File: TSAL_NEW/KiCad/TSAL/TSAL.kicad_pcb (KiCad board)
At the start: 2 copper layers, 101.6 x 25.4 mm, 0 parts

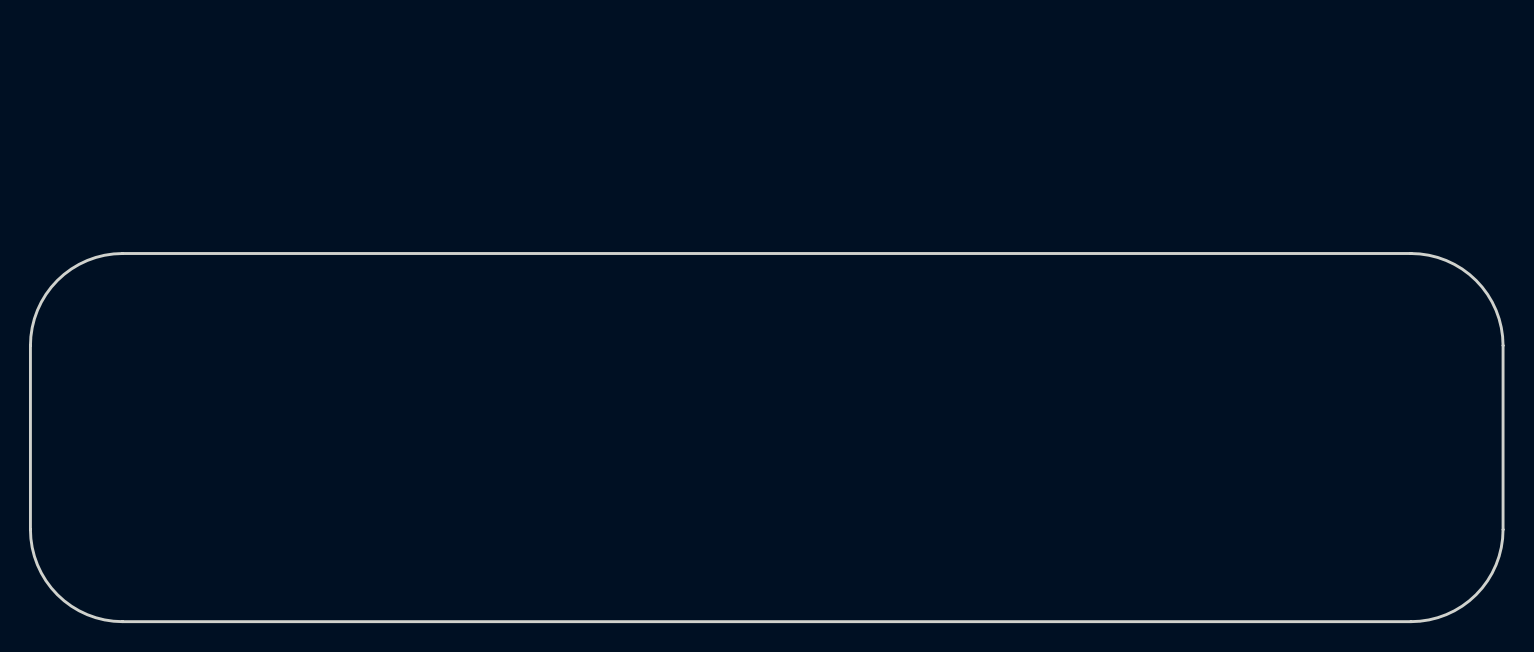
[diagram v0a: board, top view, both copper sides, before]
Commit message: Ready for Review
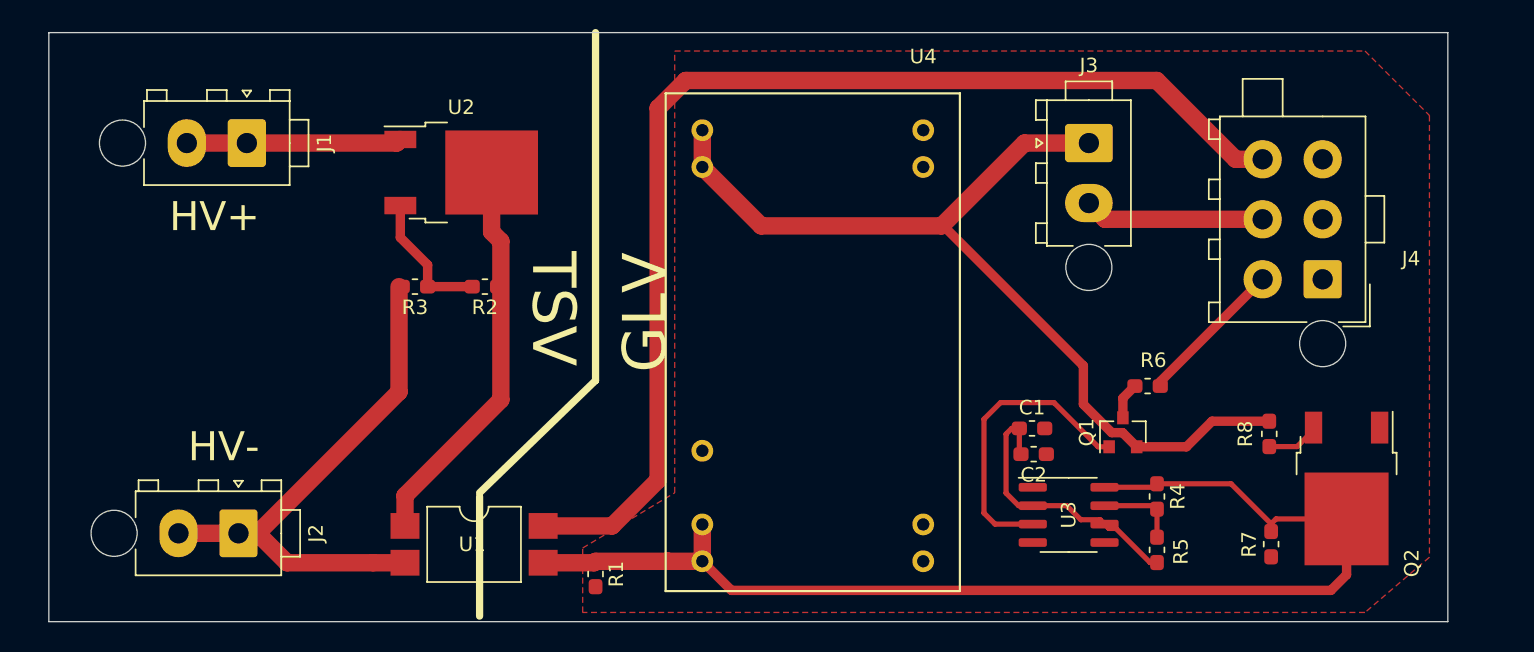
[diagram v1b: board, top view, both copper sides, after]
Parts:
- added C1: 1u, Capacitor_SMD:C_0603_1608Metric_Pad1.05x0.95mm_HandSolder, F.Cu at (174.5, 113.7)
- added C2: 1u, Capacitor_SMD:C_0603_1608Metric_Pad1.05x0.95mm_HandSolder, F.Cu at (174.6, 115.4)
- added J1: HV INPUT, Connector_TE-Connectivity:TE_MATE-N-LOK_1-770866-x_1x02_P4.14mm_Vertical, F.Cu at (120.3, 94.0)
- added J2: HV GND, Connector_TE-Connectivity:TE_MATE-N-LOK_1-770866-x_1x02_P4.14mm_Vertical, F.Cu at (119.8, 120.9)
- added J3: Green_LED_Jp, Connector_TE-Connectivity:TE_MATE-N-LOK_1-770866-x_1x02_P4.14mm_Vertical, F.Cu at (178.4, 94.0)
- added J4: Conn_02x03_Counter_Clockwise, Connector_TE-Connectivity:TE_MATE-N-LOK_1-770875-x_2x03_P4.14mm_Vertical, F.Cu at (194.6, 103.4)
- added Q1: BSS84, Package_TO_SOT_SMD:SOT-23, F.Cu at (180.8, 113.9)
- added Q2: FDD8447L, Package_TO_SOT_SMD:TO-252-2, F.Cu at (196.2, 117.8)
- added R1: 10k, Resistor_SMD:R_0603_1608Metric_Pad1.05x0.95mm_HandSolder, F.Cu at (144.4, 123.7)
- added R2: 180k, Resistor_SMD:R_0603_1608Metric_Pad1.05x0.95mm_HandSolder, F.Cu at (136.8, 103.9)
- added R3: 20k, Resistor_SMD:R_0603_1608Metric_Pad1.05x0.95mm_HandSolder, F.Cu at (131.9, 103.9)
- added R4: 100k, Resistor_SMD:R_0603_1608Metric_Pad1.05x0.95mm_HandSolder, F.Cu at (183.1, 118.4)
- added R5: 235k, Resistor_SMD:R_0603_1608Metric_Pad1.05x0.95mm_HandSolder, F.Cu at (183.1, 122.0)
- added R6: R, Resistor_SMD:R_0603_1608Metric_Pad1.05x0.95mm_HandSolder, F.Cu at (182.5, 110.7)
- added R7: 10k, Resistor_SMD:R_0603_1608Metric_Pad1.05x0.95mm_HandSolder, F.Cu at (191.0, 121.7)
- added R8: 1k, Resistor_SMD:R_0603_1608Metric_Pad1.05x0.95mm_HandSolder, F.Cu at (190.9, 114.0)
- added U1: LTV-817S, Package_DIP:SMDIP-4_W9.53mm, F.Cu at (136.0, 121.7)
- added U2: LR8K4-G, Package_TO_SOT_SMD:TO-252-2, F.Cu at (135.1, 96.0)
- added U3: LM555, Package_SO:SOIC-8_3.9x4.9mm_P1.27mm, F.Cu at (177.0, 119.6)
- added U4: LDB-350L, aero_footprint:LDB-_L, F.Cu at (167.0, 93.1)
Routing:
- net +12V: track 0.00 -> 81.8 mm
- net /GLV+: track 0.00 -> 79.7 mm
- net +24V: track 0.00 -> 64.5 mm
- net GNDA: track 0.00 -> 38.0 mm
- net +12VA: track 0.00 -> 27.4 mm
- net /555_OUTPUT: track 0.00 -> 20.5 mm
- net /THR: track 0.00 -> 19.4 mm
- net /HV+: track 0.00 -> 14.8 mm
- net /LED_GREEN+: track 0.00 -> 12.5 mm
- net /LED_RED+: track 0.00 -> 10.3 mm
- net Net-(R2-Pad2): track 0.00 -> 9.45 mm
- net /DIS: track 0.00 -> 5.65 mm
- net Net-(Q2-Pad3): track 0.00 -> 3.70 mm
- net Net-(Q1-Pad3): track 0.00 -> 2.53 mm
- added copper zone on F.Cu, net GND
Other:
- board size 101.6 x 25.4 mm -> 96.5 x 40.6 mm
- net class HV added: clearance 0.85, trace_width 1.2, via_dia 1, via_drill 0.6
- board text added: "GLV"
- board text added: "HV+"
- board text added: "HV-"
- board text added: "TSV"
